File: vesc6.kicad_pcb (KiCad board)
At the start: 4 copper layers, 70 x 60 mm, 126 parts, among them J1 Main, J2 HALL_ENC, J6 USB, Q1 DMN62D0UW, Q2 HYG015N10NS1TA, Q3 HYG015N10NS1TA, Q4 HYG015N10NS1TA, Q5 HYG015N10NS1TA, Q6 HYG015N10NS1TA, Q7 HYG015N10NS1TA, SW1 SENS_VOLTAGE, U1 STM32F405RGTx, U10 AD8418, U11 Mc74VHC1GT66, U12 AD8418, U14 SN65HVD232, U2 Mc74VHC1GT66, U3 DRV8301DCAR, U4 Mc74VHC1GT66, U5 Mc74VHC1GT66, U6 TLV73333PDBV, U7 AD8418, U8 Mc74VHC1GT66, U9 Mc74VHC1GT66, Y1 8M

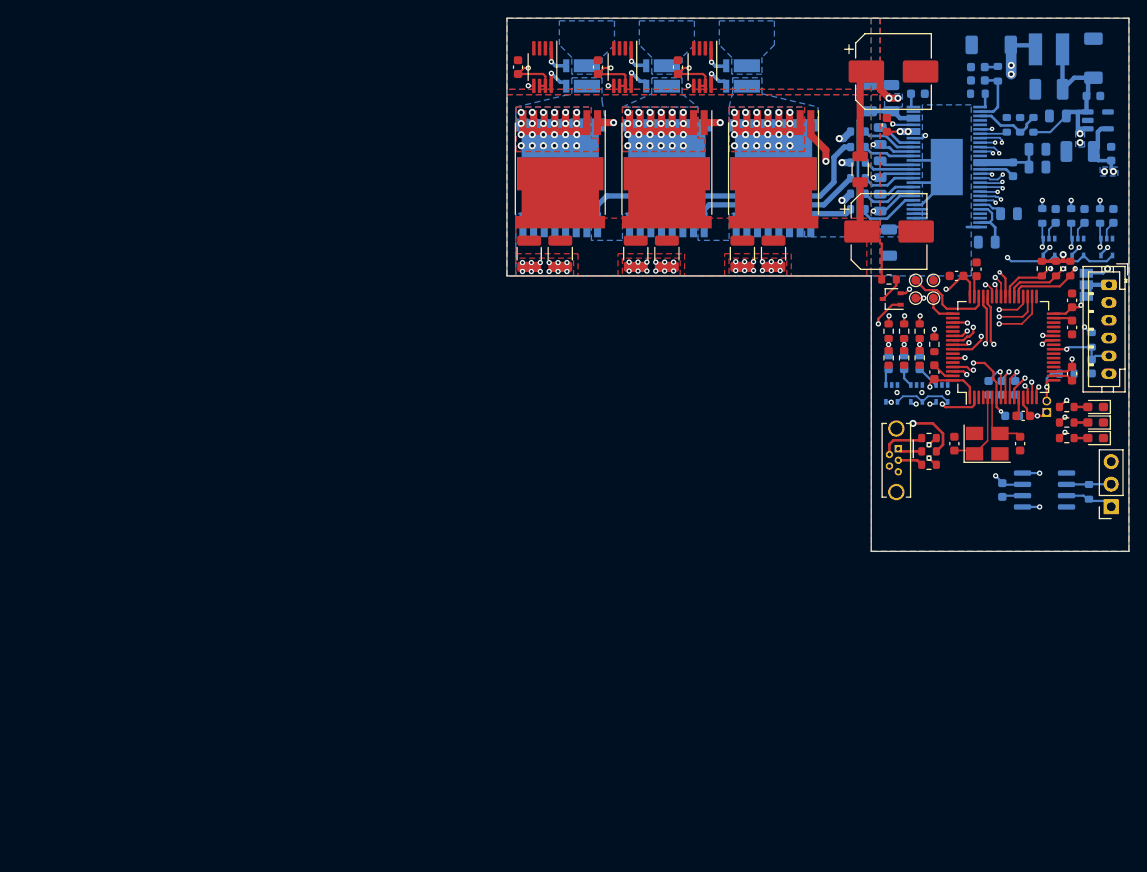
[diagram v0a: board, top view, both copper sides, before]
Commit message: Update
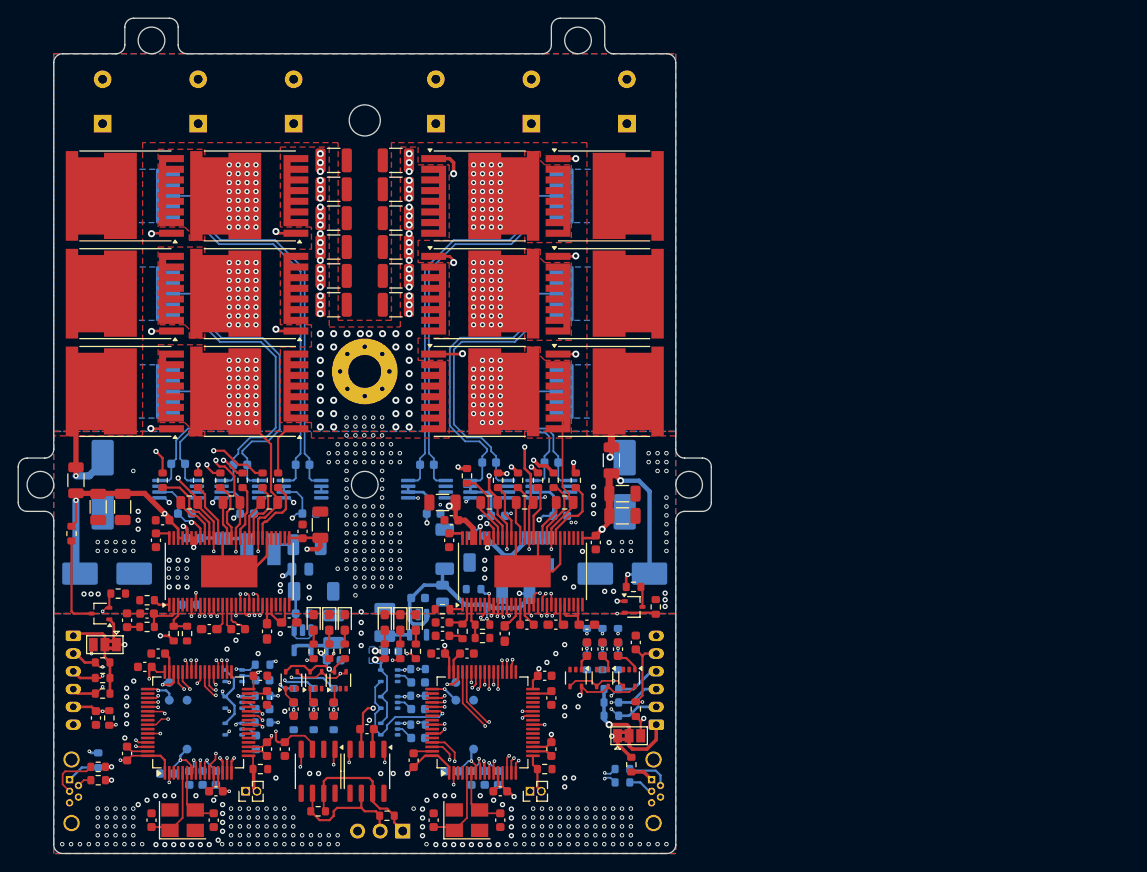
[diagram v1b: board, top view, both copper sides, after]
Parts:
- added C1: 100n, Capacitor_SMD:C_0603_1608Metric, F.Cu at (161.0, 85.0)
- added C100: 15n, Capacitor_SMD:C_0603_1608Metric, F.Cu at (111.5, 84.8)
- added C101: 100n, Capacitor_SMD:C_0603_1608Metric, F.Cu at (131.5, 103.8)
- added C102: 100n, Capacitor_SMD:C_0603_1608Metric, B.Cu at (115.8, 84.5)
- added C103: 220n, Capacitor_SMD:C_0805_2012Metric, F.Cu at (115.2, 80.5)
- added C104: 220n, Capacitor_SMD:C_0805_2012Metric, F.Cu at (120.0, 80.5)
- added C105: 220n, Capacitor_SMD:C_0805_2012Metric, F.Cu at (124.2, 80.5)
- added C106: 100n, Capacitor_SMD:C_0603_1608Metric, F.Cu at (128.0, 83.8)
- added C107: 4.7u, Capacitor_SMD:C_1206_3216Metric, F.Cu at (130.0, 83.0)
- added C108: 100n, Capacitor_SMD:C_0603_1608Metric, F.Cu at (112.2, 82.5)
- added C109: 4.7u, Capacitor_SMD:C_1206_3216Metric, F.Cu at (107.8, 81.0)
- added C110: 4.7u, Capacitor_SMD:C_1206_3216Metric, F.Cu at (105.0, 81.0)
- added C111: 2.2u, Capacitor_SMD:C_0805_2012Metric, B.Cu at (127.8, 88.0)
- added C112: 22u, Capacitor_SMD:CP_Elec_8x6.2, B.Cu at (106.0, 88.5)
- added C113: 100u, Capacitor_Tantalum_SMD:CP_EIA-3528-21_Kemet-B, B.Cu at (128.5, 85.2)
- added C114: 100n, Capacitor_SMD:C_0603_1608Metric, B.Cu at (128.0, 93.0)
- added C115: 22u, Capacitor_SMD:CP_Elec_8x6.2, B.Cu at (105.5, 78.5)
- added C116: 100n, Capacitor_SMD:C_0603_1608Metric, B.Cu at (131.5, 98.2)
- added C117: 100u, Capacitor_Tantalum_SMD:CP_EIA-3528-21_Kemet-B, B.Cu at (131.5, 94.8)
- added C118: 100n, Capacitor_SMD:C_0603_1608Metric, F.Cu at (126.0, 108.2)
- added C2: 100n, Capacitor_SMD:C_0603_1608Metric, F.Cu at (144.8, 82.5)
- added C4: 100n, Capacitor_SMD:C_0603_1608Metric, F.Cu at (104.8, 104.8)
- added C43: 470u, Capacitor_THT:CP_Radial_D10.0mm_P5.00mm, B.Cu at (143.0, 37.9)
- added C45: 470u, Capacitor_THT:CP_Radial_D10.0mm_P5.00mm, B.Cu at (153.8, 37.9)
- added C47: 470u, Capacitor_THT:CP_Radial_D10.0mm_P5.00mm, B.Cu at (164.5, 37.9)
- added C59: 100n, Capacitor_SMD:C_0603_1608Metric, B.Cu at (128.8, 81.8)
- added C60: 15n, Capacitor_SMD:C_0603_1608Metric, B.Cu at (123.5, 100.5)
- added C61: 1n, Capacitor_SMD:C_0603_1608Metric, B.Cu at (142.0, 76.2)
- added C62: 1n, Capacitor_SMD:C_0603_1608Metric, B.Cu at (149.0, 76.0)
- added C63: 1n, Capacitor_SMD:C_0603_1608Metric, B.Cu at (156.0, 76.0)
- added C64: 1n, Capacitor_SMD:C_0603_1608Metric, B.Cu at (115.2, 111.5)
- added C65: 4.7u, Capacitor_SMD:C_1210_3225Metric, F.Cu at (131.5, 58.2)
- added C66: 4.7u, Capacitor_SMD:C_1210_3225Metric, F.Cu at (131.5, 55.0)
- added C67: 470u, Capacitor_THT:CP_Radial_D10.0mm_P5.00mm, B.Cu at (105.5, 37.9)
- added C68: 1n, Capacitor_SMD:C_0603_1608Metric, B.Cu at (121.0, 76.2)
- added C69: 100n, Capacitor_SMD:C_0603_1608Metric, B.Cu at (121.8, 81.8)
- added C70: 470u, Capacitor_THT:CP_Radial_D10.0mm_P5.00mm, B.Cu at (116.2, 37.9)
- added C71: 15n, Capacitor_SMD:C_0603_1608Metric, B.Cu at (123.5, 103.8)
- added C72: 470u, Capacitor_THT:CP_Radial_D10.0mm_P5.00mm, B.Cu at (127.0, 37.9)
- added C73: 1n, Capacitor_SMD:C_0603_1608Metric, B.Cu at (116.8, 111.5)
- added C74: 4.7u, Capacitor_SMD:C_1210_3225Metric, F.Cu at (131.5, 51.8)
- added C75: 4.7u, Capacitor_SMD:C_1210_3225Metric, F.Cu at (131.5, 48.5)
- added C76: 1n, Capacitor_SMD:C_0603_1608Metric, B.Cu at (114.0, 76.2)
- added C77: 100n, Capacitor_SMD:C_0603_1608Metric, B.Cu at (114.8, 81.8)
- added C78: 15n, Capacitor_SMD:C_0603_1608Metric, B.Cu at (122.8, 107.5)
- added C79: 1n, Capacitor_SMD:C_0603_1608Metric, B.Cu at (118.2, 111.5)
- added C80: 4.7u, Capacitor_SMD:C_1210_3225Metric, F.Cu at (131.5, 45.2)
- added C81: 4.7u, Capacitor_SMD:C_1210_3225Metric, F.Cu at (131.5, 42.0)
- added C82: 100n, Capacitor_SMD:C_0603_1608Metric, F.Cu at (108.2, 108.8)
- added C83: 100n, Capacitor_SMD:C_0603_1608Metric, F.Cu at (118.2, 113.0)
- added C84: 100n, Capacitor_SMD:C_0603_1608Metric, F.Cu at (124.0, 108.2)
- added C85: 100n, Capacitor_SMD:C_0603_1608Metric, F.Cu at (110.2, 99.0)
- added C86: 100n, Capacitor_SMD:C_0603_1608Metric, F.Cu at (123.2, 100.0)
- added C87: 15p, Capacitor_SMD:C_0603_1608Metric, F.Cu at (111.0, 116.2)
- added C88: 15p, Capacitor_SMD:C_0603_1608Metric, F.Cu at (118.0, 116.2)
- added C89: 100n, Capacitor_SMD:C_0603_1608Metric, B.Cu at (112.8, 111.0)
- added C90: 1u, Capacitor_SMD:C_0603_1608Metric, F.Cu at (124.0, 102.5)
- added C91: 1u, Capacitor_SMD:C_0603_1608Metric, F.Cu at (111.8, 97.5)
- added C92: 2.2u, Capacitor_SMD:C_0603_1608Metric_Pad1.08x0.95mm_HandSolder, F.Cu at (117.5, 94.8)
- added C93: 6n8, Capacitor_SMD:C_0603_1608Metric, F.Cu at (108.2, 93.8)
- added C94: 100n, Capacitor_SMD:C_0603_1608Metric, F.Cu at (127.0, 103.8)
- added C95: 22n, Capacitor_SMD:C_0603_1608Metric, F.Cu at (120.8, 94.8)
- added C96: 2.2u, Capacitor_SMD:C_0603_1608Metric_Pad1.08x0.95mm_HandSolder, F.Cu at (124.0, 95.0)
- added C97: 120p, Capacitor_SMD:C_0603_1608Metric, F.Cu at (110.5, 93.0)
- added C98: 2.2u, Capacitor_SMD:C_0603_1608Metric_Pad1.08x0.95mm_HandSolder, F.Cu at (126.5, 94.0)
- added C99: 100n, Capacitor_SMD:C_0603_1608Metric, F.Cu at (129.2, 103.8)
- added D1: GRN, LED_SMD:LED_0603_1608Metric_Pad1.05x0.95mm_HandSolder, F.Cu at (129.2, 94.0)
- added D10: 5V, Diode_SMD:D_SOD-128, B.Cu at (129.2, 90.5)
- added D2: RED, LED_SMD:LED_0603_1608Metric_Pad1.05x0.95mm_HandSolder, F.Cu at (131.0, 94.0)
- added D3: BLU, LED_SMD:LED_0603_1608Metric_Pad1.05x0.95mm_HandSolder, F.Cu at (132.8, 94.0)
- added D4: D_Schottky, Diode_SMD:D_SOD-128, B.Cu at (119.0, 86.8)
- added FB2: FerriteBead, Resistor_SMD:R_1206_3216Metric, F.Cu at (102.5, 78.0)
- added H1: MountingHole_Pad, MountingHole:MountingHole_3.7mm_Pad_Via, F.Cu at (135.0, 65.8)
- added J3: HALL_ENC, Connector_JST:JST_PH_B6B-PH-K_1x06_P2.00mm_Vertical, B.Cu at (102.2, 95.5)
- added J4: USB, Connector_USB:USB_Micro-B_Wuerth_614105150721_Vertical_CircularHoles, B.Cu at (101.8, 111.7)
- added L2: 22u, Inductor_SMD:L_Bourns-SRN4018, B.Cu at (123.2, 85.8)
- added Q10: HYG015N10NS1TA, Package_TO_SOT_SMD:Infineon_PG-HSOF-8-1, F.Cu at (108.0, 57.0)
- added Q11: HYG015N10NS1TA, Package_TO_SOT_SMD:Infineon_PG-HSOF-8-1, F.Cu at (122.0, 57.0)
- added Q12: HYG015N10NS1TA, Package_TO_SOT_SMD:Infineon_PG-HSOF-8-1, F.Cu at (108.0, 68.0)
- added Q13: HYG015N10NS1TA, Package_TO_SOT_SMD:Infineon_PG-HSOF-8-1, F.Cu at (122.0, 68.0)
- added Q14: DMN62D0UW, Package_TO_SOT_SMD:SOT-323_SC-70, F.Cu at (105.2, 93.0)
- added Q8: HYG015N10NS1TA, Package_TO_SOT_SMD:Infineon_PG-HSOF-8-1, F.Cu at (108.0, 46.0)
- added Q9: HYG015N10NS1TA, Package_TO_SOT_SMD:Infineon_PG-HSOF-8-1, F.Cu at (122.0, 46.0)
- added R1: 0.5m, TUWR_Sensors:WSLP3921, B.Cu at (153.0, 46.0)
- added R2: 0.5m, TUWR_Sensors:WSLP3921, B.Cu at (153.0, 57.0)
- added R3: 0.5m, TUWR_Sensors:WSLP3921, B.Cu at (153.0, 68.0)
- added R4: 2.2k, Resistor_SMD:R_0603_1608Metric, F.Cu at (105.5, 98.5)
- added R44: 22, Resistor_SMD:R_0603_1608Metric, F.Cu at (105.0, 111.8)
- added R45: 220, Resistor_SMD:R_0603_1608Metric, F.Cu at (129.2, 97.2)
- added R46: 220, Resistor_SMD:R_0603_1608Metric, F.Cu at (131.0, 97.2)
- added R47: 1k, Resistor_SMD:R_0603_1608Metric, F.Cu at (132.8, 97.2)
- added R48: 10k, Resistor_SMD:R_0603_1608Metric, F.Cu at (123.2, 110.5)
- added R49: 0.5m, TUWR_Sensors:WSLP3921, B.Cu at (117.0, 68.0)
- added R5: 2.2k, Resistor_SMD:R_0603_1608Metric, F.Cu at (105.5, 100.2)
- added R50: 4.7, Resistor_SMD:R_0603_1608Metric, F.Cu at (112.2, 78.0)
- added R51: 4.7, Resistor_SMD:R_0603_1608Metric, F.Cu at (116.2, 78.0)
- added R52: 1k, Resistor_SMD:R_0603_1608Metric, B.Cu at (123.5, 98.8)
- added R53: 0.5m, TUWR_Sensors:WSLP3921, B.Cu at (117.0, 57.0)
- added R54: 4.7, Resistor_SMD:R_0603_1608Metric, F.Cu at (118.8, 78.0)
- added R55: 4.7, Resistor_SMD:R_0603_1608Metric, F.Cu at (121.2, 78.0)
- added R56: 1k, Resistor_SMD:R_0603_1608Metric, B.Cu at (123.5, 102.2)
- added R57: 0.5m, TUWR_Sensors:WSLP3921, B.Cu at (117.0, 46.0)
- added R58: 1k, Resistor_SMD:R_0603_1608Metric, B.Cu at (123.5, 105.2)
- added R59: 4.7, Resistor_SMD:R_0603_1608Metric, F.Cu at (123.5, 78.0)
- added R60: 4.7, Resistor_SMD:R_0603_1608Metric, F.Cu at (125.2, 78.0)
- added R61: 3.3k, Resistor_SMD:R_0603_1608Metric, F.Cu at (115.0, 95.2)
- added R62: 18k, Resistor_SMD:R_0603_1608Metric, F.Cu at (113.5, 95.2)
- added R63: 15k, Resistor_SMD:R_0603_1608Metric, F.Cu at (110.5, 94.5)
- added R64: 39k, Resistor_SMD:R_0603_1608Metric, B.Cu at (127.0, 102.2)
- added R65: 2.2k, Resistor_SMD:R_0603_1608Metric, B.Cu at (127.0, 105.2)
- added R66: 220k, Resistor_SMD:R_0603_1608Metric, F.Cu at (110.5, 91.5)
- added R67: 10k, Resistor_SMD:R_0603_1608Metric, B.Cu at (115.2, 92.0)
- added R68: 39k, Resistor_SMD:R_0603_1608Metric, B.Cu at (129.2, 102.2)
- added R69: 2.2k, Resistor_SMD:R_0603_1608Metric, B.Cu at (129.2, 105.2)
- added R70: 39k, Resistor_SMD:R_0603_1608Metric, B.Cu at (131.5, 102.2)
- added R71: 2.2k, Resistor_SMD:R_0603_1608Metric, B.Cu at (131.5, 105.2)
- added R72: 39K, Resistor_SMD:R_0603_1608Metric, F.Cu at (102.0, 84.0)
- added R73: 2.2k, Resistor_SMD:R_0603_1608Metric, F.Cu at (107.2, 90.8)
- added R74: 120, Resistor_SMD:R_0603_1608Metric, F.Cu at (129.8, 115.2)
- added R9: 2.2k, Resistor_SMD:R_0603_1608Metric, F.Cu at (105.5, 102.0)
- added SW2: SENS_VOLTAGE, Jumper:SolderJumper-3_P1.3mm_Bridged2Bar12_Pad1.0x1.5mm, F.Cu at (105.8, 96.5)
- added TH2: NTC, Connector_PinHeader_1.27mm:PinHeader_1x02_P1.27mm_Vertical, F.Cu at (121.6, 113.0)
- added TP5: SWCLK, TestPoint:TestPoint_Pad_D1.0mm, B.Cu at (113.0, 102.8)
- added TP6: SWDIO, TestPoint:TestPoint_Pad_D1.0mm, B.Cu at (113.0, 100.8)
- added TP7: NRST, TestPoint:TestPoint_Pad_D1.0mm, B.Cu at (115.0, 108.2)
- added TP8: GND, TestPoint:TestPoint_Pad_D1.0mm, B.Cu at (115.0, 102.8)
- added U13: AD8418, Package_SO:MSOP-8_3x3mm_P0.65mm, B.Cu at (128.0, 79.0)
- added U15: Mc74VHC1GT66, Package_TO_SOT_SMD:SOT-353_SC-70-5, B.Cu at (120.2, 100.0)
- added U16: Mc74VHC1GT66, Package_TO_SOT_SMD:SOT-353_SC-70-5, B.Cu at (120.2, 103.0)
- added U17: AD8418, Package_SO:MSOP-8_3x3mm_P0.65mm, B.Cu at (121.0, 79.0)
- added U18: Mc74VHC1GT66, Package_TO_SOT_SMD:SOT-353_SC-70-5, B.Cu at (120.2, 106.0)
- added U19: AD8418, Package_SO:MSOP-8_3x3mm_P0.65mm, B.Cu at (114.0, 79.0)
- added U20: STM32F405RGTx, Package_QFP:LQFP-64_10x10mm_P0.5mm, F.Cu at (116.2, 105.2)
- added U21: Mc74VHC1GT66, Package_TO_SOT_SMD:SOT-353_SC-70-5, F.Cu at (126.8, 100.5)
- added U22: DRV8301DCAR, Package_SO:HTSSOP-56-1EP_6.1x14mm_P0.5mm_EP3.61x6.35mm, F.Cu at (119.8, 88.2)
- added U23: Mc74VHC1GT66, Package_TO_SOT_SMD:SOT-353_SC-70-5, F.Cu at (129.5, 100.5)
- added U24: Mc74VHC1GT66, Package_TO_SOT_SMD:SOT-353_SC-70-5, F.Cu at (132.2, 100.5)
- added U25: TLV73333PDBV, Package_TO_SOT_SMD:SOT-23-5, B.Cu at (128.0, 96.0)
- added U26: SN65HVD232, Package_SO:SOIC-8_3.9x4.9mm_P1.27mm, F.Cu at (129.8, 110.8)
- added Y2: 8M, Crystal:Crystal_SMD_EuroQuartz_MT-4Pin_3.2x2.5mm_HandSoldering, F.Cu at (114.5, 116.2)
- C15, C19, C20, C22, C23, C24, C25, C26, C28, C29, C3, C30, C31, C32, C57, Q3, Q5, Q7, R11, R17, R18, R19, R22, R30, R32, R33, R36, R37, R41, R42, R43, SW1, U14, U2, U3, U4, U5: moved to F.Cu
- C16: value 2.2u -> 1n; footprint Capacitor_SMD:C_0805_2012Metric -> Capacitor_SMD:C_0603_1608Metric
- C17, C18, C21: footprint Capacitor_SMD:C_0805_2012Metric -> Capacitor_SMD:C_0603_1608Metric_Pad1.08x0.95mm_HandSolder; moved to F.Cu
- C27, C56, C58, J1, J2, J6, R12, R13, R20, R21, R24, R25, R26, R27, R6, R7, R8, TP1, TP2, TP3, TP4, U10, U12, U7: moved to B.Cu
- C35, C36: value 2.2u -> 100n
- C38, C44, C51: value 2.2u -> 100n; moved to B.Cu
- R31: value 0.5m -> 0; footprint TUWR_Sensors:BVN_1216 -> Resistor_SMD:R_0603_1608Metric
- R35: value 0.5m -> 10k; footprint TUWR_Sensors:BVN_1216 -> Resistor_SMD:R_0603_1608Metric; moved to F.Cu
- R39: value 0.5m -> 22; footprint TUWR_Sensors:BVN_1216 -> Resistor_SMD:R_0603_1608Metric; moved to F.Cu
- moved R39 106.6 mm to (105.0, 110.2)
- moved C36 98.5 mm to (138.0, 97.2), turned to 0 degrees
- moved R35 95.7 mm to (106.2, 104.8), turned to -90 degrees
- moved U6 95.3 mm to (141.0, 94.2), turned to -90 degrees
- moved C35 94.7 mm to (141.0, 91.2)
- moved R31 94.6 mm to (105.0, 109.5), turned to 90 degrees
- moved C37 94.5 mm to (137.2, 94.0), turned to 90 degrees
- moved C39 94.2 mm to (141.0, 100.8), turned to 180 degrees
- moved U8 94.1 mm to (137.8, 100.0), turned to 180 degrees
- moved C46 93.3 mm to (141.0, 103.8), turned to 180 degrees
- moved U9 92.9 mm to (137.8, 103.0), turned to 180 degrees
- moved C52 92.7 mm to (141.0, 107.0), turned to 180 degrees
- moved R34 92.1 mm to (141.0, 99.2), turned to 0 degrees
- moved U11 92.0 mm to (137.8, 106.0), turned to 180 degrees
- moved D9 91.6 mm to (144.0, 85.8)
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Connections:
- net /VESC_Right/CAN/RX renamed /VESC_Left/CAN/RX
- net /VESC_Right/CAN/TX renamed /VESC_Left/CAN/TX
- net /VESC_Right/CAN_H renamed /VESC_Left/CAN_H
- net /VESC_Right/CAN_L renamed /VESC_Left/CAN_L
- net /VESC_Right/DRV8301/CS renamed /VESC_Left/DRV8301/CS
- net /VESC_Right/DRV8301/EN_GATE renamed /VESC_Left/DRV8301/EN_GATE
- net /VESC_Right/DRV8301/FAULT renamed /VESC_Left/DRV8301/FAULT
- net /VESC_Right/DRV8301/GH_A renamed /VESC_Left/DRV8301/GH_A
- net /VESC_Right/DRV8301/GH_B renamed /VESC_Left/DRV8301/GH_B
- net /VESC_Right/DRV8301/GH_C renamed /VESC_Left/DRV8301/GH_C
- net /VESC_Right/DRV8301/GL_A renamed /VESC_Left/DRV8301/GL_A
- net /VESC_Right/DRV8301/GL_B renamed /VESC_Left/DRV8301/GL_B
- net /VESC_Right/DRV8301/GL_C renamed /VESC_Left/DRV8301/GL_C
- net /VESC_Right/DRV8301/INH_A renamed /VESC_Left/DRV8301/INH_A
- net /VESC_Right/DRV8301/INH_B renamed /VESC_Left/DRV8301/INH_B
- net /VESC_Right/DRV8301/INH_C renamed /VESC_Left/DRV8301/INH_C
- net /VESC_Right/DRV8301/INL_A renamed /VESC_Left/DRV8301/INL_A
- net /VESC_Right/DRV8301/INL_B renamed /VESC_Left/DRV8301/INL_B
- net /VESC_Right/DRV8301/INL_C renamed /VESC_Left/DRV8301/INL_C
- net /VESC_Right/DRV8301/SCLK renamed /VESC_Left/DRV8301/SCLK
- net /VESC_Right/DRV8301/SENS_A renamed /VESC_Left/DRV8301/SENS_A
- net /VESC_Right/DRV8301/SENS_B renamed /VESC_Left/DRV8301/SENS_B
- net /VESC_Right/DRV8301/SENS_C renamed /VESC_Left/DRV8301/SENS_C
- net /VESC_Right/DRV8301/SENS_FILTERED renamed /VESC_Left/DRV8301/SENS_FILTERED
- net /VESC_Right/DRV8301/SENS_SUPPLY renamed /VESC_Left/DRV8301/SENS_SUPPLY
- net /VESC_Right/EN_BUCK renamed /VESC_Left/EN_BUCK
- net /VESC_Right/MCU/ADC_15 renamed /VESC_Left/MCU/ADC_15
- net /VESC_Right/MCU/ADC_TEMP renamed /VESC_Left/MCU/ADC_TEMP
- net /VESC_Right/MCU/CURRENT_1 renamed /VESC_Left/MCU/CURRENT_1
- net /VESC_Right/MCU/CURRENT_2 renamed /VESC_Left/MCU/CURRENT_2
- net /VESC_Right/MCU/CURRENT_3 renamed /VESC_Left/MCU/CURRENT_3
- net /VESC_Right/MCU/CURR_FILTER_ON renamed /VESC_Left/MCU/CURR_FILTER_ON
- net /VESC_Right/MCU/HALL_1 renamed /VESC_Left/MCU/HALL_1
- net /VESC_Right/MCU/HALL_2 renamed /VESC_Left/MCU/HALL_2
- net /VESC_Right/MCU/HALL_3 renamed /VESC_Left/MCU/HALL_3
- net /VESC_Right/MCU/LED_GREEN renamed /VESC_Left/MCU/LED_GREEN
- net /VESC_Right/MCU/LED_RED renamed /VESC_Left/MCU/LED_RED
- net /VESC_Right/MCU/MISO_ADC_EXT2 renamed /VESC_Left/MCU/MISO_ADC_EXT2
- net /VESC_Right/MCU/NRST renamed /VESC_Left/MCU/NRST
- net /VESC_Right/MCU/RX_SDA_NSS renamed /VESC_Left/MCU/RX_SDA_NSS
- net /VESC_Right/MCU/SCK_ADC_EXT renamed /VESC_Left/MCU/SCK_ADC_EXT
- net /VESC_Right/MCU/SERVO renamed /VESC_Left/MCU/SERVO
- net /VESC_Right/MCU/SWCLK renamed /VESC_Left/MCU/SWCLK
- net /VESC_Right/MCU/SWDIO renamed /VESC_Left/MCU/SWDIO
- net /VESC_Right/MCU/TX_SCL_MOSI renamed /VESC_Left/MCU/TX_SCL_MOSI
- net /VESC_Right/MCU/USB_D_N renamed /VESC_Left/MCU/USB_D_N
- net /VESC_Right/Power/C_A renamed /VESC_Left/Power_alternate/C_A
- net /VESC_Right/Power/C_B renamed /VESC_Left/Power_alternate/C_B
- net /VESC_Right/Power/C_C renamed /VESC_Left/Power_alternate/C_C
- C16 pad 1: Net-(U3-CP1) -> /VESC_Right/Power/SH_A_P
- C16 pad 2: GND -> /VESC_Right/Power/SH_A_N
- C17 pad 1: Net-(U3-CP1) -> Net-(U3-GVDD)
- C25 pad 1: /VESC_Right/DRV8301/Supply_Filterted -> /VESC_Left/DRV8301/Supply_Filterted
- C28 pad 1: /VESC_Right/SH_A -> /VESC_Left/Power_alternate/SH_A_P
- C29 pad 1: /VESC_Right/DRV8301/SH_B -> /VESC_Left/Power_alternate/SH_B_P
- C3 pad 1: /VESC_Right/MCU/TEMP_MOTOR -> /VESC_Left/MCU/TEMP_MOTOR
- C30 pad 1: /VESC_Right/DRV8301/SH_C -> /VESC_Left/Power_alternate/SH_C_P
- C31 pad 1: /VESC_Right/DRV8301/Supply_Filterted -> /VESC_Left/DRV8301/Supply_Filterted
- C32 pad 1: /VESC_Right/DRV8301/Supply_Filterted -> /VESC_Left/DRV8301/Supply_Filterted
- C33 pad 1: /VESC_Right/5V -> /VESC_Left/5V
- C34 pad 1: /VESC_Right/5V -> /VESC_Left/5V
- C35 pad 1: /VESC_Right/5V -> /VESC_Left/5V
- C36 pad 1: /VESC_Right/3.3V -> /VESC_Left/3.3V
- C37 pad 1: /VESC_Right/3.3V -> /VESC_Left/3.3V
- C38 pad 2: /VESC_Right/3.3V -> /VESC_Left/3.3V
- C41 pad 1: /VESC_Right/DRV8301/SUPPLY -> /VESC_Left/SUPPLY
- C42 pad 1: /VESC_Right/DRV8301/SUPPLY -> /VESC_Left/SUPPLY
- C44 pad 2: /VESC_Right/3.3V -> /VESC_Left/3.3V
- C49 pad 1: /VESC_Right/DRV8301/SUPPLY -> /VESC_Left/SUPPLY
- C5 pad 1: /VESC_Right/3.3V -> /VESC_Left/3.3V
- C50 pad 1: /VESC_Right/DRV8301/SUPPLY -> /VESC_Left/SUPPLY
- C51 pad 2: /VESC_Right/3.3V -> /VESC_Left/3.3V
- C54 pad 1: /VESC_Right/DRV8301/SUPPLY -> /VESC_Left/SUPPLY
- C55 pad 1: /VESC_Right/DRV8301/SUPPLY -> /VESC_Left/SUPPLY
- C56 pad 1: /VESC_Right/DRV8301/SUPPLY -> /VESC_Left/SUPPLY
- C57 pad 1: /VESC_Right/3.3V -> /VESC_Left/3.3V
- C58 pad 1: /VESC_Right/DRV8301/Supply_Filterted -> /VESC_Left/DRV8301/Supply_Filterted
- C6 pad 1: /VESC_Right/3.3V -> /VESC_Left/3.3V
- C7 pad 1: /VESC_Right/3.3V -> /VESC_Left/3.3V
- C8 pad 1: /VESC_Right/3.3V -> /VESC_Left/3.3V
- C9 pad 1: /VESC_Right/3.3V -> /VESC_Left/3.3V
- D9 pad 2: /VESC_Right/5V -> /VESC_Left/5V
- FB1 pad 1: /VESC_Right/DRV8301/Supply_Filterted -> /VESC_Left/DRV8301/Supply_Filterted
- FB1 pad 2: /VESC_Right/DRV8301/SUPPLY -> /VESC_Left/SUPPLY
- J2 pad 5: /VESC_Right/MCU/TEMP_MOTOR -> /VESC_Left/MCU/TEMP_MOTOR
- L1 pad 2: /VESC_Right/5V -> /VESC_Left/5V
- Q1 pad 1: /VESC_Right/5V -> /VESC_Left/5V
- Q2 pad 2: /VESC_Right/SH_A -> /VESC_Left/Power_alternate/SH_A_P
- Q2 pad 3: /VESC_Right/DRV8301/SUPPLY -> /VESC_Left/SUPPLY
- Q3 pad 3: /VESC_Right/SH_A -> /VESC_Left/Power_alternate/SH_A_P
- Q4 pad 1: /VESC_Right/DRV8301/SH_C -> Net-(Q4-G)
- Q4 pad 2: /VESC_Right/DRV8301/SH_B -> /VESC_Left/Power_alternate/SH_B_P
- Q4 pad 3: /VESC_Right/DRV8301/SUPPLY -> /VESC_Left/SUPPLY
- Q5 pad 3: /VESC_Right/DRV8301/SH_B -> /VESC_Left/Power_alternate/SH_B_P
- Q6 pad 2: /VESC_Right/DRV8301/SH_C -> /VESC_Left/Power_alternate/SH_C_P
- Q6 pad 3: /VESC_Right/DRV8301/SUPPLY -> /VESC_Left/SUPPLY
- Q7 pad 3: /VESC_Right/DRV8301/SH_C -> /VESC_Left/Power_alternate/SH_C_P
- R10 pad 2: /VESC_Right/5V -> /VESC_Left/5V
- R11 pad 1: /VESC_Right/MCU/TEMP_MOTOR -> /VESC_Left/MCU/TEMP_MOTOR
- R11 pad 2: /VESC_Right/3.3V -> /VESC_Left/3.3V
- R12 pad 2: /VESC_Right/MCU/USB_D_P -> /VESC_Left/MCU/USB_D_P
- R16 pad 2: /VESC_Right/3.3V -> /VESC_Left/3.3V
- R18 pad 2: /VESC_Right/5V -> /VESC_Left/5V
- R20 pad 1: /VESC_Right/SH_A -> /VESC_Left/Power_alternate/SH_A_P
- R24 pad 1: /VESC_Right/DRV8301/SH_B -> /VESC_Left/Power_alternate/SH_B_P
- R26 pad 1: /VESC_Right/DRV8301/SH_C -> /VESC_Left/Power_alternate/SH_C_P
- R28 pad 1: /VESC_Right/DRV8301/SUPPLY -> /VESC_Left/DRV8301/Supply_Filterted
- R31 pad 1: /VESC_Right/SH_A -> Net-(J4-VBUS)
- R31 pad 2: Net-(U7-IN+) -> /VESC_Right/5V
- R35 pad 1: /VESC_Right/DRV8301/SH_B -> /VESC_Right/MCU/TEMP_MOTOR
- R35 pad 2: Net-(U10-IN+) -> /VESC_Right/3.3V
- R36 pad 2: /VESC_Right/DRV8301/SH_C -> Net-(Q4-G)
- R39 pad 1: /VESC_Right/DRV8301/SH_C -> Net-(J4-D+)
- R39 pad 2: Net-(U12-IN+) -> /VESC_Right/MCU/USB_D_P
- SW1 pad 1: /VESC_Right/3.3V -> /VESC_Left/5V
- SW1 pad 3: /VESC_Right/5V -> /VESC_Left/3.3V
- TH1 pad 1: /VESC_Right/3.3V -> /VESC_Left/3.3V
- U1 pad 1: /VESC_Right/3.3V -> /VESC_Left/3.3V
- U1 pad 13: /VESC_Right/3.3V -> /VESC_Left/3.3V
- U1 pad 19: /VESC_Right/3.3V -> /VESC_Left/3.3V
- U1 pad 24: /VESC_Right/MCU/TEMP_MOTOR -> /VESC_Left/MCU/TEMP_MOTOR
- U1 pad 32: /VESC_Right/3.3V -> /VESC_Left/3.3V
- U1 pad 45: /VESC_Right/MCU/USB_D_P -> /VESC_Left/MCU/USB_D_P
- U1 pad 48: /VESC_Right/3.3V -> /VESC_Left/3.3V
- U1 pad 52: unconnected-(U1-PC11-Pad52) -> /VESC_Left/DRV8301/SDO
- U1 pad 53: unconnected-(U1-PC12-Pad53) -> /VESC_Left/DRV8301/SDI
- U1 pad 55: /VESC_Right/DRV8301/SDO -> unconnected-(U1-PB3-Pad55)
- U1 pad 56: /VESC_Right/DRV8301/SDI -> unconnected-(U1-PB4-Pad56)
- U1 pad 64: /VESC_Right/3.3V -> /VESC_Left/3.3V
- U10 pad 1: Net-(U10-IN-) -> /VESC_Left/Power_alternate/SH_B_N
- U10 pad 6: /VESC_Right/3.3V -> /VESC_Left/3.3V
- U10 pad 7: /VESC_Right/3.3V -> /VESC_Left/3.3V
- U10 pad 8: Net-(U10-IN+) -> /VESC_Left/Power_alternate/SH_B_P
- U11 pad 5: /VESC_Right/3.3V -> /VESC_Left/3.3V
- U12 pad 1: Net-(U12-IN-) -> /VESC_Left/Power_alternate/SH_C_N
- U12 pad 6: /VESC_Right/3.3V -> /VESC_Left/3.3V
- U12 pad 7: /VESC_Right/3.3V -> /VESC_Left/3.3V
- U12 pad 8: Net-(U12-IN+) -> /VESC_Left/Power_alternate/SH_C_P
- U14 pad 3: /VESC_Right/3.3V -> /VESC_Left/3.3V
- U2 pad 5: /VESC_Right/3.3V -> /VESC_Left/3.3V
- U3 pad 10: /VESC_Right/DRV8301/SDO -> /VESC_Left/DRV8301/SDO
- U3 pad 13: Net-(U3-CP1) -> Net-(U3-GVDD)
- U3 pad 29: /VESC_Right/DRV8301/Supply_Filterted -> /VESC_Left/DRV8301/Supply_Filterted
- U3 pad 36: /VESC_Right/DRV8301/SH_C -> /VESC_Left/Power_alternate/SH_C_P
- U3 pad 41: /VESC_Right/DRV8301/SH_B -> /VESC_Left/Power_alternate/SH_B_P
- U3 pad 46: /VESC_Right/SH_A -> /VESC_Left/Power_alternate/SH_A_P
- U3 pad 49: /VESC_Right/3.3V -> /VESC_Left/3.3V
- U3 pad 53: /VESC_Right/DRV8301/Supply_Filterted -> /VESC_Left/DRV8301/Supply_Filterted
- U3 pad 54: /VESC_Right/DRV8301/Supply_Filterted -> /VESC_Left/DRV8301/Supply_Filterted
- U3 pad 9: /VESC_Right/DRV8301/SDI -> /VESC_Left/DRV8301/SDI
- U4 pad 5: /VESC_Right/3.3V -> /VESC_Left/3.3V
- U5 pad 5: /VESC_Right/3.3V -> /VESC_Left/3.3V
- U6 pad 1: /VESC_Right/5V -> /VESC_Left/5V
- U6 pad 3: /VESC_Right/5V -> /VESC_Left/5V
- U6 pad 5: /VESC_Right/3.3V -> /VESC_Left/3.3V
- U7 pad 1: Net-(U7-IN-) -> /VESC_Left/Power_alternate/SH_A_N
- U7 pad 6: /VESC_Right/3.3V -> /VESC_Left/3.3V
- U7 pad 7: /VESC_Right/3.3V -> /VESC_Left/3.3V
- U7 pad 8: Net-(U7-IN+) -> /VESC_Left/Power_alternate/SH_A_P
- U8 pad 5: /VESC_Right/3.3V -> /VESC_Left/3.3V
- U9 pad 5: /VESC_Right/3.3V -> /VESC_Left/3.3V
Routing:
- net /VESC_Right/Power/SH_A_P: track 0.00 -> 119.3 mm, vias 0 -> 35
- net /VESC_Left/Power_alternate/SH_A_P: track 0.00 -> 112.4 mm, vias 0 -> 35
- net /VESC_Left/3.3V: track 0.00 -> 104.5 mm, vias 0 -> 14
- net /VESC_Right/Power/SH_B_P: track 0.00 -> 93.4 mm, vias 0 -> 35
- net /VESC_Left/Power_alternate/SH_B_P: track 0.00 -> 81.9 mm, vias 0 -> 35
- net /VESC_Right/SH_A: track 75.5 -> 0.00 mm, vias 26 -> 0
- net /VESC_Left/5V: track 0.00 -> 64.4 mm, vias 0 -> 4
- net /VESC_Left/Power_alternate/C_A: track 85.5 -> 21.2 mm
- net /VESC_Right/DRV8301/SH_C: track 57.2 -> 0.00 mm, vias 28 -> 0
- net /VESC_Right/Power/SH_C_P: track 0.00 -> 56.0 mm, vias 0 -> 34
- net /VESC_Left/DRV8301/Supply_Filterted: track 0.00 -> 54.2 mm, vias 0 -> 4
- net /VESC_Right/DRV8301/SH_B: track 53.0 -> 0.00 mm, vias 26 -> 0
- net /VESC_Left/Power_alternate/SH_C_P: track 0.00 -> 47.8 mm, vias 0 -> 32
- net /VESC_Left/Power_alternate/C_B: track 72.2 -> 25.8 mm
- net /VESC_Left/Power_alternate/SH_A_N: track 0.00 -> 45.2 mm
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- added copper zone on B.Cu, net /VESC_Left/3.3V
- added copper zone on In1.Cu, net /VESC_Left/3.3V
- added copper zone on B.Cu, net /VESC_Left/Power_alternate/SH_A_N
- added copper zone on B.Cu, net /VESC_Left/Power_alternate/SH_A_P
- added copper zone on F.Cu, net /VESC_Left/Power_alternate/SH_A_P
- added copper zone on In1.Cu, net /VESC_Left/Power_alternate/SH_A_P
- added copper zone on In2.Cu, net /VESC_Left/Power_alternate/SH_A_P
- added copper zone on B.Cu, net /VESC_Left/Power_alternate/SH_B_N
- added copper zone on B.Cu, net /VESC_Left/Power_alternate/SH_B_P
- added copper zone on F.Cu, net /VESC_Left/Power_alternate/SH_B_P
- added copper zone on In1.Cu, net /VESC_Left/Power_alternate/SH_B_P
- added copper zone on In2.Cu, net /VESC_Left/Power_alternate/SH_B_P
- added copper zone on B.Cu, net /VESC_Left/Power_alternate/SH_C_N
- added copper zone on B.Cu, net /VESC_Left/Power_alternate/SH_C_P
- added copper zone on F.Cu, net /VESC_Left/Power_alternate/SH_C_P
- added copper zone on In1.Cu, net /VESC_Left/Power_alternate/SH_C_P
- added copper zone on In2.Cu, net /VESC_Left/Power_alternate/SH_C_P
- added copper zone on F.Cu, net /VESC_Left/SUPPLY
- added copper zone on In1.Cu, net /VESC_Right/3.3V
- added copper zone on B.Cu, net /VESC_Right/Power/SH_A_N
- added copper zone on B.Cu, net /VESC_Right/Power/SH_A_P
- added copper zone on F.Cu, net /VESC_Right/Power/SH_A_P
- added copper zone on In1.Cu, net /VESC_Right/Power/SH_A_P
- added copper zone on In2.Cu, net /VESC_Right/Power/SH_A_P
- added copper zone on B.Cu, net /VESC_Right/Power/SH_B_N
- added copper zone on B.Cu, net /VESC_Right/Power/SH_B_P
- added copper zone on F.Cu, net /VESC_Right/Power/SH_B_P
- added copper zone on In1.Cu, net /VESC_Right/Power/SH_B_P
- added copper zone on In2.Cu, net /VESC_Right/Power/SH_B_P
- added copper zone on B.Cu, net /VESC_Right/Power/SH_C_N
- added copper zone on B.Cu, net /VESC_Right/Power/SH_C_P
- added copper zone on F.Cu, net /VESC_Right/Power/SH_C_P
- added copper zone on In1.Cu, net /VESC_Right/Power/SH_C_P
- added copper zone on In2.Cu, net /VESC_Right/Power/SH_C_P
- removed copper zone on B.Cu, net /VESC_Right/3.3V
- removed copper zone on In2.Cu, net /VESC_Right/3.3V
- removed copper zone on B.Cu, net /VESC_Right/5V
- removed copper zone on B.Cu, net /VESC_Right/DRV8301/SH_B
- removed copper zone on F.Cu, net /VESC_Right/DRV8301/SH_B
- removed copper zone on In1.Cu, net /VESC_Right/DRV8301/SH_B
- removed copper zone on In2.Cu, net /VESC_Right/DRV8301/SH_B
- removed copper zone on B.Cu, net /VESC_Right/DRV8301/SH_C
- removed copper zone on F.Cu, net /VESC_Right/DRV8301/SH_C
- removed copper zone on In1.Cu, net /VESC_Right/DRV8301/SH_C
- removed copper zone on In2.Cu, net /VESC_Right/DRV8301/SH_C
- removed copper zone on F.Cu, net /VESC_Right/DRV8301/SUPPLY
- removed copper zone on B.Cu, net /VESC_Right/DRV8301/Supply_Filterted
- removed copper zone on B.Cu, net /VESC_Right/Power/PH_A
- removed copper zone on B.Cu, net /VESC_Right/Power/PH_B
- removed copper zone on B.Cu, net /VESC_Right/Power/PH_C
- removed copper zone on B.Cu, net /VESC_Right/SH_A
- removed copper zone on F.Cu, net /VESC_Right/SH_A
- removed copper zone on In1.Cu, net /VESC_Right/SH_A
- removed copper zone on In2.Cu, net /VESC_Right/SH_A
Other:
- board size 70 x 60 mm -> 78 x 94 mm
